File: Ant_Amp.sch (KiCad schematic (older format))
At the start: 23 parts, among them Q1 BF981

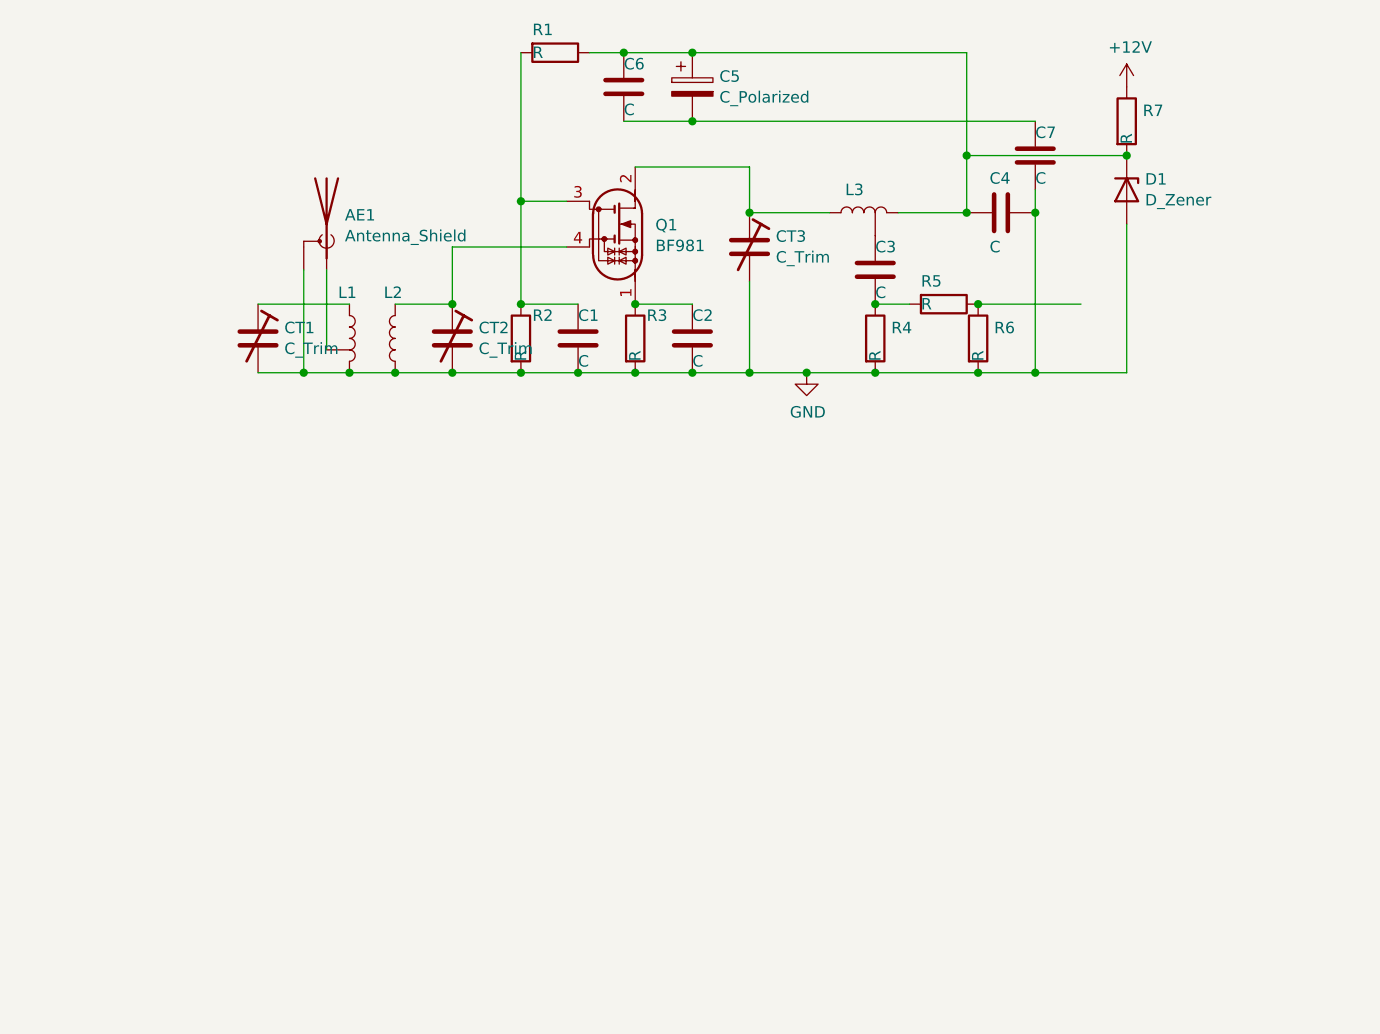
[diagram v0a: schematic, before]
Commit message: :qw
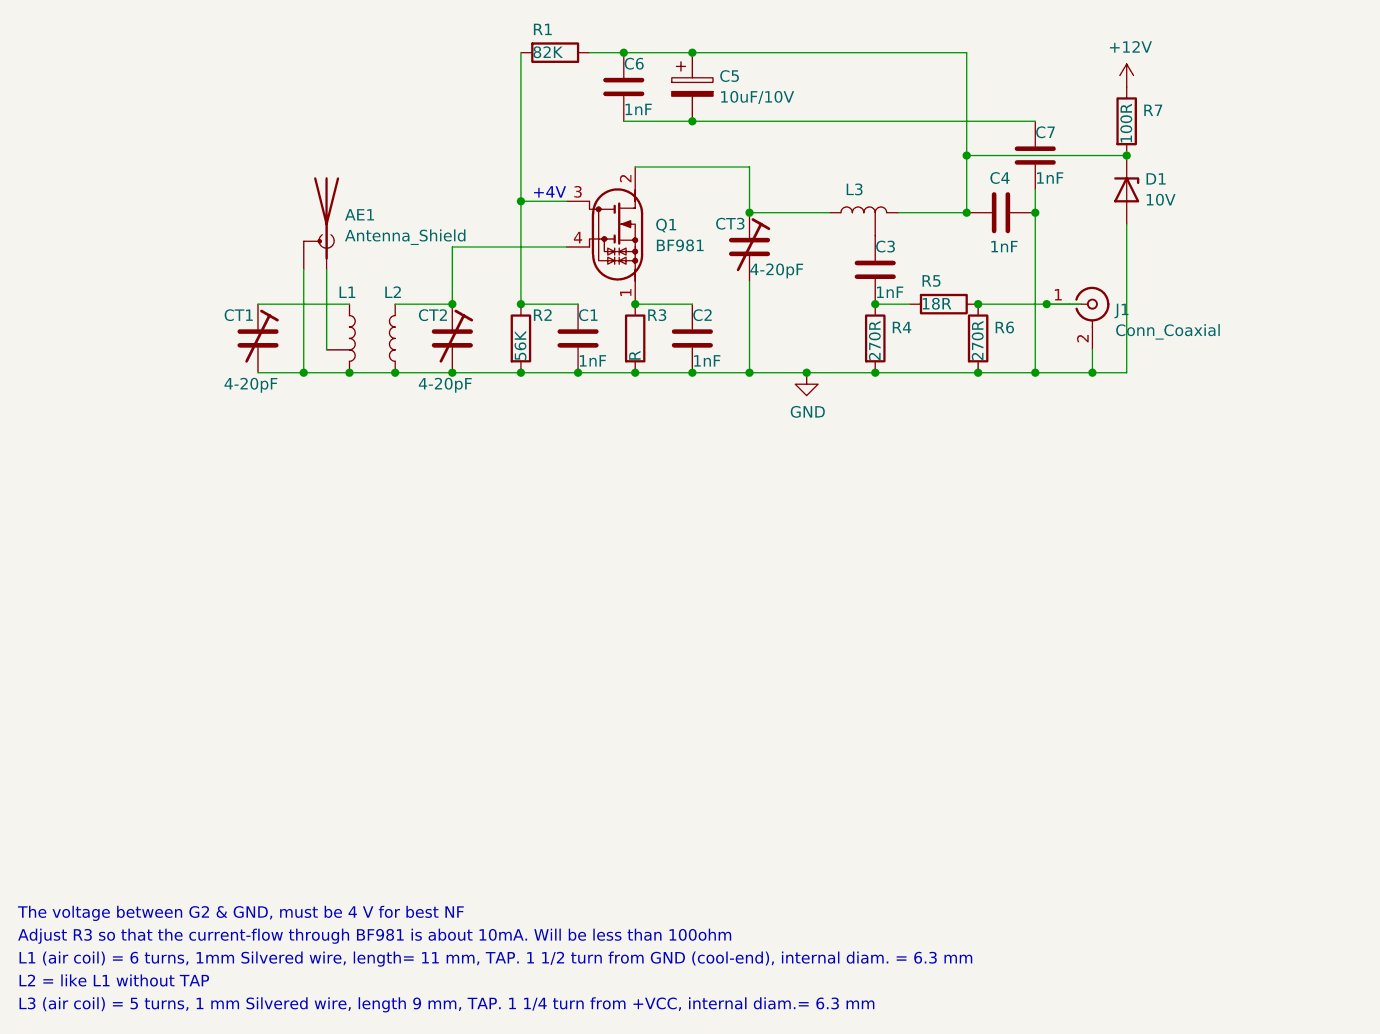
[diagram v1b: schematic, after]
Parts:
- added J1: Conn_Coaxial, Connector2:Urydell_SMA_Haaks, symbol Connector:Conn_Coaxial
- AE1: footprint (none) -> Connector2:Urydell_SMA_Haaks
- C1, C2, C4, C6, C7: value C -> 1nF
- C3: value C -> 1nF; footprint (none) -> Capacitor_SMD:C_0603_1608Metric
- C5: value C_Polarized -> 10uF/10V; footprint (none) -> Capacitor_SMD:C_1206_3216Metric
- CT1, CT2, CT3: value C_Trim -> 4-20pF; footprint (none) -> Capacitor_SMD:C_Trimmer_Voltronics_JR
- D1: value D_Zener -> 10V; footprint (none) -> Diode_SMD:D_SMA
- L1, L3: footprint (none) -> Inductor:L_6T_11mm_intdiam6.3mm_1mm_wire_tap1.5T
- L2: footprint (none) -> Inductor:L_6T_11mm_intdiam6.3mm_1mm_wire
- R1: value R -> 82K
- R2: value R -> 56K
- R4, R6: value R -> 270R
- R5: value R -> 18R
- R7: value R -> 100R
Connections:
- net GND: now also J1.2 (Ext)
- net at R5.1, R6.1: now also J1.1 (In)
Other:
- note added: "+4V"
- note added: "Adjust R3 so that the current-flow through BF981 is about 10mA. Will be less than 100ohm"
- note added: "L1 (air coil) = 6 turns, 1mm Silvered wire, length= 11 mm, TAP. 1 1/2 turn from GND (cool-end), internal diam. = 6.3 mm"
- note added: "L2 = like L1 without TAP"
- note added: "L3 (air coil) = 5 turns, 1 mm Silvered wire, length 9 mm, TAP. 1 1/4 turn from +VCC, internal diam.= 6.3 mm\n"
- note added: "The voltage between G2 & GND, must be 4 V for best NF"
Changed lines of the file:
@@
 F 0 "AE1" H 2420 2689 50  0000 R CNN
 F 1 "Antenna_Shield" H 2420 2598 50  0000 R CNN
-F 2 "" H 2500 2750 50  0001 C CNN
+F 2 "Connector2:Urydell_SMA_Haaks" H 2500 2750 50  0001 C CNN
 F 3 "~" H 2500 2750 50  0001 C CNN
 	1    2500 2650
@@
 F 0 "L2" H 2850 2950 50  0000 R CNN
 F 1 "L" H 2756 3195 50  0001 R CNN
-F 2 "" H 2800 3150 50  0001 C CNN
+F 2 "Inductor:L_6T_11mm_intdiam6.3mm_1mm_wire" H 2800 3150 50  0001 C CNN
 F 3 "~" H 2800 3150 50  0001 C CNN
 	1    2800 3150
@@
 U 1 1 602959A7
 P 2200 3150
-F 0 "CT1" H 2315 3196 50  0000 L CNN
-F 1 "C_Trim" H 2315 3105 50  0000 L CNN
-F 2 "" H 2200 3150 50  0001 C CNN
+F 0 "CT1" H 2050 3250 50  0000 L CNN
+F 1 "4-20pF" H 2050 2950 50  0000 L CNN
+F 2 "Capacitor_SMD:C_Trimmer_Voltronics_JR" H 2200 3150 50  0001 C CNN
 F 3 "~" H 2200 3150 50  0001 C CNN
 	1    2200 3150
@@
 F 0 "L1" H 2550 3350 50  0000 L CNN
 F 1 "L-Tap" H 2653 3105 50  0001 L CNN
-F 2 "" H 2600 3150 50  0001 C CNN
+F 2 "Inductor:L_6T_11mm_intdiam6.3mm_1mm_wire_tap1.5T" H 2600 3150 50  0001 C CNN
 F 3 "~" H 2600 3150 50  0001 C CNN
 	1    2600 3150
@@
 U 1 1 6029D25D
 P 3050 3150
-F 0 "CT2" H 3165 3196 50  0000 L CNN
-F 1 "C_Trim" H 3165 3105 50  0000 L CNN
-F 2 "" H 3050 3150 50  0001 C CNN
+F 0 "CT2" H 2900 3250 50  0000 L CNN
+F 1 "4-20pF" H 2900 2950 50  0000 L CNN
+F 2 "Capacitor_SMD:C_Trimmer_Voltronics_JR" H 3050 3150 50  0001 C CNN
 F 3 "~" H 3050 3150 50  0001 C CNN
 	1    3050 3150
@@
 P 3350 3150
 F 0 "R2" H 3400 3250 50  0000 L CNN
-F 1 "R" V 3350 3050 50  0000 L CNN
+F 1 "56K" V 3350 3050 50  0000 L CNN
 F 2 "Resistor_SMD:R_0603_1608Metric" V 3280 3150 50  0001 C CNN
 F 3 "~" H 3350 3150 50  0001 C CNN
@@
 P 3600 3150
 F 0 "C1" H 3600 3250 50  0000 L CNN
-F 1 "C" H 3600 3050 50  0000 L CNN
+F 1 "1nF" H 3600 3050 50  0000 L CNN
 F 2 "Capacitor_SMD:C_0603_1608Metric" H 3638 3000 50  0001 C CNN
 F 3 "~" H 3600 3150 50  0001 C CNN
@@
 P 4100 3150
 F 0 "C2" H 4100 3250 50  0000 L CNN
-F 1 "C" H 4100 3050 50  0000 L CNN
+F 1 "1nF" H 4100 3050 50  0000 L CNN
 F 2 "Capacitor_SMD:C_0603_1608Metric" H 4138 3000 50  0001 C CNN
 F 3 "~" H 4100 3150 50  0001 C CNN
@@
 U 1 1 602B4533
 P 4350 2750
-F 0 "CT3" H 4465 2796 50  0000 L CNN
-F 1 "C_Trim" H 4465 2705 50  0000 L CNN
-F 2 "" H 4350 2750 50  0001 C CNN
+F 0 "CT3" H 4200 2850 50  0000 L CNN
+F 1 "4-20pF" H 4350 2650 50  0000 L CNN
+F 2 "Capacitor_SMD:C_Trimmer_Voltronics_JR" H 4350 2750 50  0001 C CNN
 F 3 "~" H 4350 2750 50  0001 C CNN
 	1    4350 2750
@@
 F 0 "L3" V 4950 2600 50  0000 L CNN
 F 1 "L-Tap" H 4903 2555 50  0001 L CNN
-F 2 "" H 4850 2600 50  0001 C CNN
+F 2 "Inductor:L_6T_11mm_intdiam6.3mm_1mm_wire_tap1.5T" H 4850 2600 50  0001 C CNN
 F 3 "~" H 4850 2600 50  0001 C CNN
 	1    4850 2600
@@
 P 4900 2850
 F 0 "C3" H 4900 2950 50  0000 L CNN
-F 1 "C" H 4900 2750 50  0000 L CNN
-F 2 "" H 4938 2700 50  0001 C CNN
+F 1 "1nF" H 4900 2750 50  0000 L CNN
+F 2 "Capacitor_SMD:C_0603_1608Metric" H 4938 2700 50  0001 C CNN
 F 3 "~" H 4900 2850 50  0001 C CNN
 	1    4900 2850
@@
 P 4900 3150
 F 0 "R4" H 4970 3196 50  0000 L CNN
-F 1 "R" V 4900 3050 50  0000 L CNN
+F 1 "270R" V 4900 3050 50  0000 L CNN
 F 2 "Resistor_SMD:R_0603_1608Metric" V 4830 3150 50  0001 C CNN
 F 3 "~" H 4900 3150 50  0001 C CNN
@@
 P 5200 3000
 F 0 "R5" V 5100 2900 50  0000 L CNN
-F 1 "R" V 5200 2900 50  0000 L CNN
+F 1 "18R" V 5200 2900 50  0000 L CNN
 F 2 "Resistor_SMD:R_0603_1608Metric" V 5130 3000 50  0001 C CNN
 F 3 "~" H 5200 3000 50  0001 C CNN
@@
 P 5350 3150
 F 0 "R6" H 5420 3196 50  0000 L CNN
-F 1 "R" V 5350 3050 50  0000 L CNN
+F 1 "270R" V 5350 3050 50  0000 L CNN
 F 2 "Resistor_SMD:R_0603_1608Metric" V 5280 3150 50  0001 C CNN
 F 3 "~" H 5350 3150 50  0001 C CNN
@@
 P 3500 1900
 F 0 "R1" V 3400 1800 50  0000 L CNN
-F 1 "R" V 3500 1800 50  0000 L CNN
+F 1 "82K" V 3500 1800 50  0000 L CNN
 F 2 "Resistor_SMD:R_0603_1608Metric" V 3430 1900 50  0001 C CNN
 F 3 "~" H 3500 1900 50  0001 C CNN
@@
 P 3800 2050
 F 0 "C6" H 3800 2150 50  0000 L CNN
-F 1 "C" H 3800 1950 50  0000 L CNN
+F 1 "1nF" H 3800 1950 50  0000 L CNN
 F 2 "Capacitor_SMD:C_0603_1608Metric" H 3838 1900 50  0001 C CNN
 F 3 "~" H 3800 2050 50  0001 C CNN
@@
 P 4100 2050
 F 0 "C5" H 4218 2096 50  0000 L CNN
-F 1 "C_Polarized" H 4218 2005 50  0000 L CNN
-F 2 "" H 4138 1900 50  0001 C CNN
+F 1 "10uF/10V" H 4218 2005 50  0000 L CNN
+F 2 "Capacitor_SMD:C_1206_3216Metric" H 4138 1900 50  0001 C CNN
 F 3 "~" H 4100 2050 50  0001 C CNN
 	1    4100 2050
@@
 P 5600 2350
 F 0 "C7" H 5600 2450 50  0000 L CNN
-F 1 "C" H 5600 2250 50  0000 L CNN
+F 1 "1nF" H 5600 2250 50  0000 L CNN
 F 2 "Capacitor_SMD:C_0603_1608Metric" H 5638 2200 50  0001 C CNN
 F 3 "~" H 5600 2350 50  0001 C CNN
@@
 P 5450 2600
 F 0 "C4" V 5300 2550 50  0000 L CNN
-F 1 "C" V 5600 2550 50  0000 L CNN
+F 1 "1nF" V 5600 2550 50  0000 L CNN
 F 2 "Capacitor_SMD:C_0603_1608Metric" H 5488 2450 50  0001 C CNN
 F 3 "~" H 5450 2600 50  0001 C CNN
@@
 P 6000 2500
 F 0 "D1" V 5954 2580 50  0000 L CNN
-F 1 "D_Zener" V 6045 2580 50  0000 L CNN
-F 2 "" H 6000 2500 50  0001 C CNN
+F 1 "10V" V 6045 2580 50  0000 L CNN
+F 2 "Diode_SMD:D_SMA" H 6000 2500 50  0001 C CNN
 F 3 "~" H 6000 2500 50  0001 C CNN
 	1    6000 2500
@@
 P 6000 2200
 F 0 "R7" H 6070 2246 50  0000 L CNN
-F 1 "R" V 6000 2100 50  0000 L CNN
+F 1 "100R" V 6000 2100 50  0000 L CNN
 F 2 "Resistor_SMD:R_0603_1608Metric" V 5930 2200 50  0001 C CNN
 F 3 "~" H 6000 2200 50  0001 C CNN
@@
 Connection ~ 5300 2600
 Wire Wire Line
-	5350 3000 5800 3000
+	6000 2650 6000 3300
+Wire Wire Line
+	6000 3300 5850 3300
+Connection ~ 5600 3300
+Text Notes 1150 5900 0    50   ~ 0
+L1 (air coil) = 6 turns, 1mm Silvered wire, length= 11 mm, TAP. 1 1/2 turn from GND (cool-end), internal diam. = 6.3 mm
+Text Notes 1150 6000 0    50   ~ 0
+L2 = like L1 without TAP
+Text Notes 1150 6100 0    50   ~ 0
+L3 (air coil) = 5 turns, 1 mm Silvered wire, length 9 mm, TAP. 1 1/4 turn from +VCC, internal diam.= 6.3 mm\n
+Text Notes 1150 5800 0    50   ~ 0
+Adjust R3 so that the current-flow through BF981 is about 10mA. Will be less than 100ohm
+Text Notes 1150 5700 0    50   ~ 0
+The voltage between G2 & GND, must be 4 V for best NF
+Text Notes 3400 2550 0    50   ~ 0
++4V
+$Comp
+L Connector:Conn_Coaxial J1
+U 1 1 602CFD53
+P 5850 3000
+F 0 "J1" H 5950 2975 50  0000 L CNN
+F 1 "Conn_Coaxial" H 5950 2884 50  0000 L CNN
+F 2 "Connector2:Urydell_SMA_Haaks" H 5850 3000 50  0001 C CNN
+F 3 " ~" H 5850 3000 50  0001 C CNN
+	1    5850 3000
+	1    0    0    -1
+$EndComp
+Wire Wire Line
+	5650 3000 5800 3000
+Wire Wire Line
+	5350 3000 5650 3000
 Connection ~ 5350 3000
-Wire Wire Line
-	6000 2650 6000 3300
-Wire Wire Line
-	6000 3300 5600 3300
-Connection ~ 5600 3300
+Connection ~ 5650 3000
+Wire Wire Line
+	5850 3200 5850 3300
+Connection ~ 5850 3300
+Wire Wire Line
+	5850 3300 5600 3300
 $EndSCHEMATC
